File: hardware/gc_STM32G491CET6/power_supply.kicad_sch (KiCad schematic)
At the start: 22 parts, among them J201 Battery, J202 Recharge, J203 USB_C_Receptacle_USB2.0, SW201 ON/OFF, U202 BU33SD5WG-TR, U203 USBLC6-2SC6, U6 AZ1117CH2-5.0TRG1

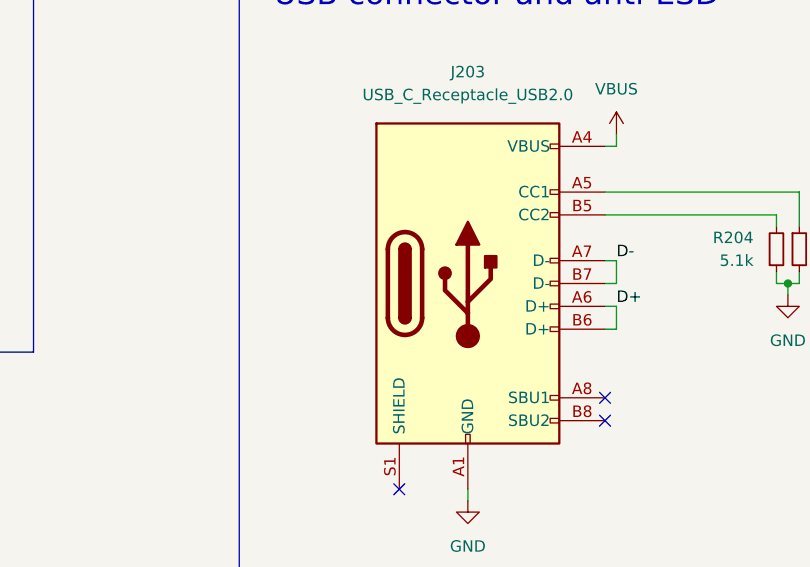
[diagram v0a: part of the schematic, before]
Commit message: silkscreen
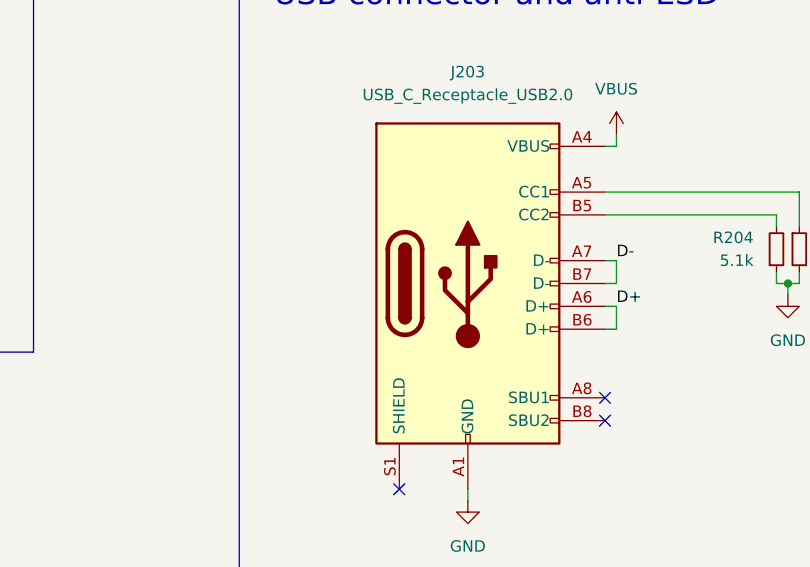
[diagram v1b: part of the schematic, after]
